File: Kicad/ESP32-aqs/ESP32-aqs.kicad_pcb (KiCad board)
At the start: 2 copper layers, 63 x 41.9 mm, 41 parts, among them IC1 CP2102N-A02-GQFN24, J1 USB4085-GF-A_REVA4, J2 JST connector SEN55, J3 ufl connector, J4 UART Connector, SW1 TC-1102-B-C-B, SW2 TC-1102-B-C-B, U1 LD1117S33TR_SOT223, U2 ESP32-WROOM-32, U3 SGP41-D-R4, U4 SX1276S8S+T-X1

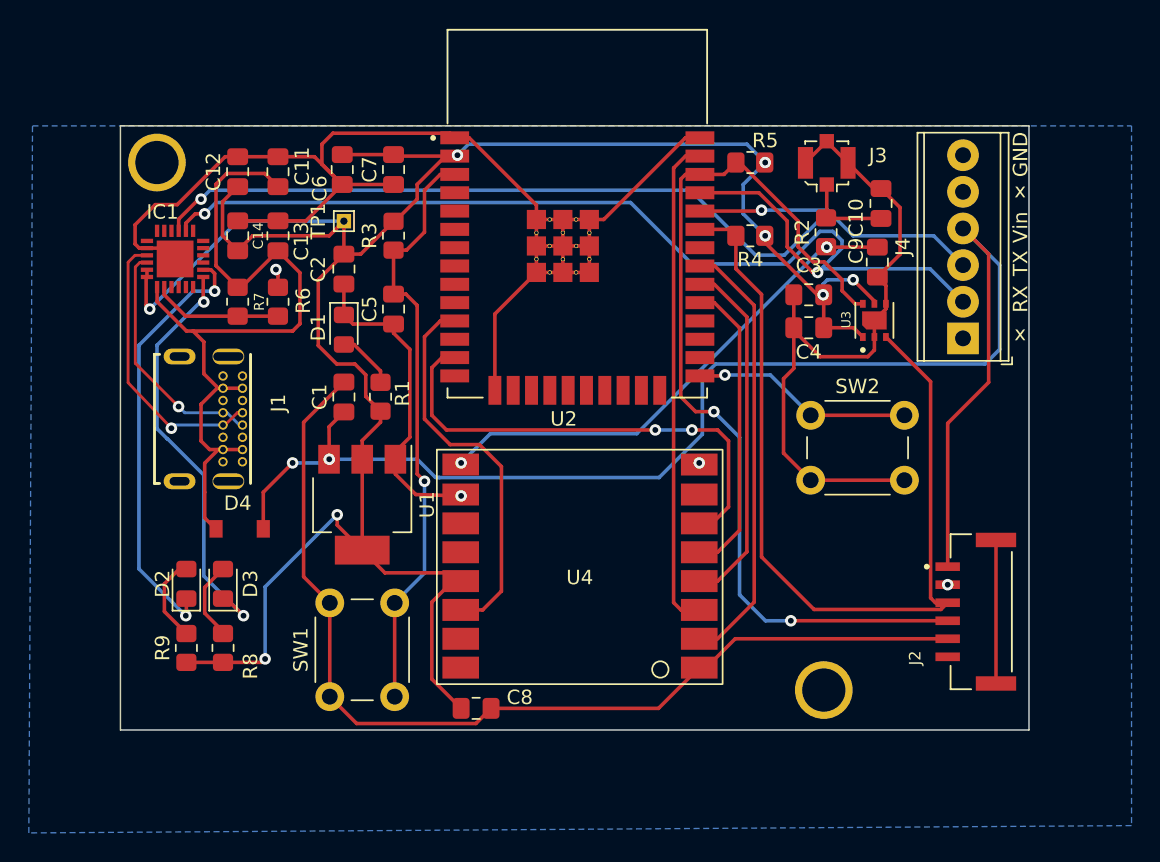
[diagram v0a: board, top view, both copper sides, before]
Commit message: pcb update
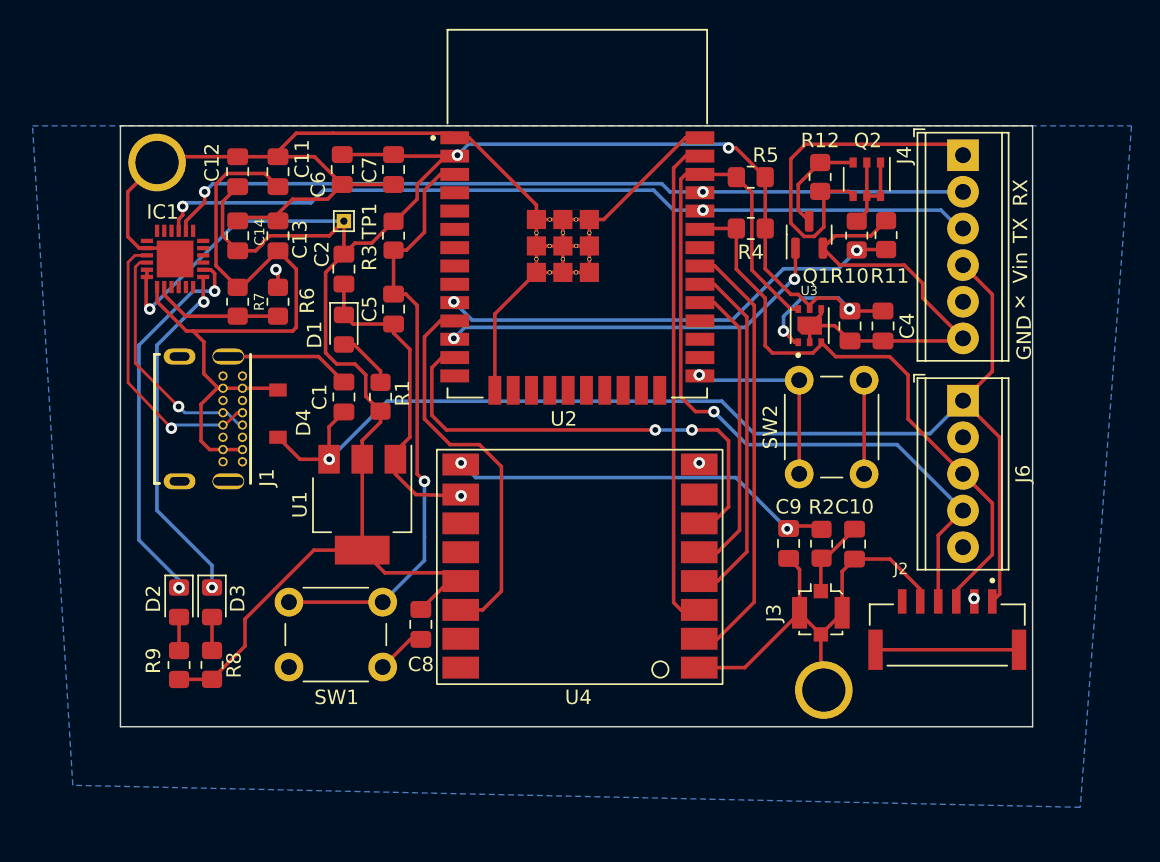
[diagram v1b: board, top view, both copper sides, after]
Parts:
- removed H4: MountingHole, MountingHole:MountingHole_2.2mm_M2_ISO7380_Pad
- added H1: MountingHole_Pad, MountingHole:MountingHole_2.2mm_M2_ISO7380_Pad, F.Cu at (127.5, 68.6)
- added J6: test point / jst connector, TerminalBlock_Phoenix:TerminalBlock_Phoenix_MPT-0,5-5-2.54_1x05_P2.54mm_Horizontal, F.Cu at (183.4, 85.1)
- added Q1: IRLML0030, Package_TO_SOT_SMD:SOT-23, F.Cu at (172.7, 73.6)
- added Q2: PMN48XP, Package_SO:TSOP-6_1.65x3.05mm_P0.95mm, F.Cu at (176.7, 69.7)
- added R10: 100k, Resistor_SMD:R_0805_2012Metric_Pad1.20x1.40mm_HandSolder, F.Cu at (176.0, 73.6)
- added R11: 100k, Resistor_SMD:R_0805_2012Metric_Pad1.20x1.40mm_HandSolder, F.Cu at (178.1, 73.6)
- added R12: 1M, Resistor_SMD:R_0805_2012Metric_Pad1.20x1.40mm_HandSolder, F.Cu at (173.5, 69.6)
- H2: value MountingHole -> MountingHole_Pad
- moved J3 31.2 mm to (173.5, 99.8), turned to 180 degrees
- moved C10 23.7 mm to (175.9, 95.0), turned to 90 degrees
- moved R2 21.6 mm to (173.6, 95.0), turned to -90 degrees
- moved C9 20.5 mm to (171.3, 95.0)
- moved J4 12.7 mm to (183.4, 68.1), turned to -90 degrees
- moved D4 8.42 mm to (135.9, 86.0), turned to -90 degrees
- moved C8 6.97 mm to (145.8, 100.6), turned to -90 degrees
- moved C4 5.15 mm to (177.8, 79.9), turned to -90 degrees
- moved U3 4.50 mm to (172.8, 79.9)
- moved J2 4.29 mm to (182.3, 102.4), turned to 0 degrees
- moved SW1 4.20 mm to (143.2, 103.6), turned to 180 degrees
- moved SW2 4.14 mm to (172.0, 90.2), turned to 90 degrees
- moved C3 3.59 mm to (175.6, 79.9), turned to -90 degrees
- moved D3 1.49 mm to (131.3, 99.1), turned to -90 degrees
- moved R8 1.40 mm to (131.3, 103.4)
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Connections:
- H2 pad 1: (no net) -> GND
- J4 pad 1: unconnected-(J4-Pin_1-Pad1) -> BAT
- U2 pad 10: unconnected-(U2-IO25-Pad10) -> VBAT
- U2 pad 12: unconnected-(U2-IO27-Pad12) -> READ_BAT
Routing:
- net VBAT: track 0.00 -> 32.6 mm, vias 0 -> 2
- net GND: track 237.7 -> 205.1 mm
- net READ_BAT: track 0.00 -> 27.5 mm, vias 0 -> 2
- net BAT: track 0.00 -> 25.1 mm
- net SDA: track 61.0 -> 42.1 mm
- net RX: track 75.1 -> 56.3 mm
- net VIN: track 99.7 -> 82.0 mm, vias 2 -> 1
- net TX: track 69.8 -> 57.5 mm
- net +3V3: track 162.9 -> 153.9 mm, vias 8 -> 5
- net ANT: track 35.1 -> 27.3 mm
- net Net-(Q2-D-Pad1): track 0.00 -> 7.62 mm
- net Net-(Q1-D): track 0.00 -> 7.30 mm
- net RXLED: track 29.4 -> 24.6 mm
- net SCL: track 65.1 -> 60.3 mm, vias 2 -> 1
- net VBUS: track 54.8 -> 50.6 mm
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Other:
- board size 63 x 41.9 mm -> 63.2 x 41.7 mm
